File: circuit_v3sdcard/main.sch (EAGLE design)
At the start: 20 parts, among them CN1 SD, CN3 MICROSD, CN4 5035481020, IC1 C8051F381-GM, IC3 N25Q512A, IC4 KC2016K, IC6 MPU-9250

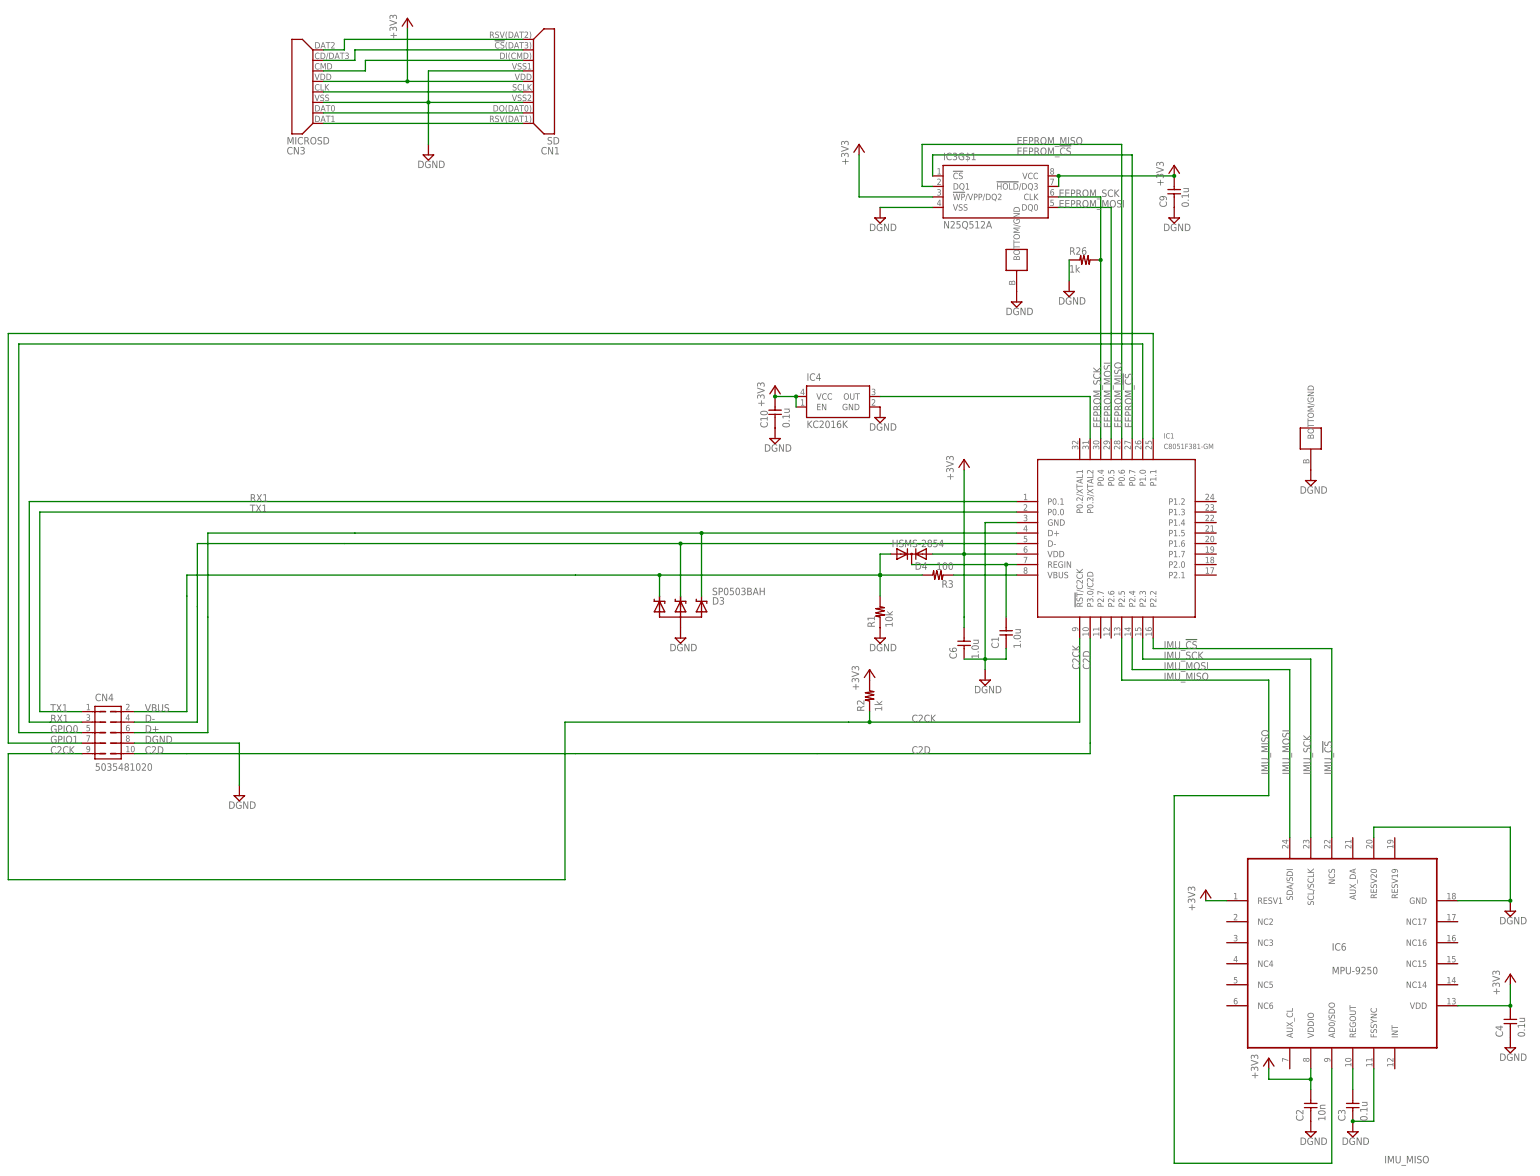
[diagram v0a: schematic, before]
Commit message: Added wiring
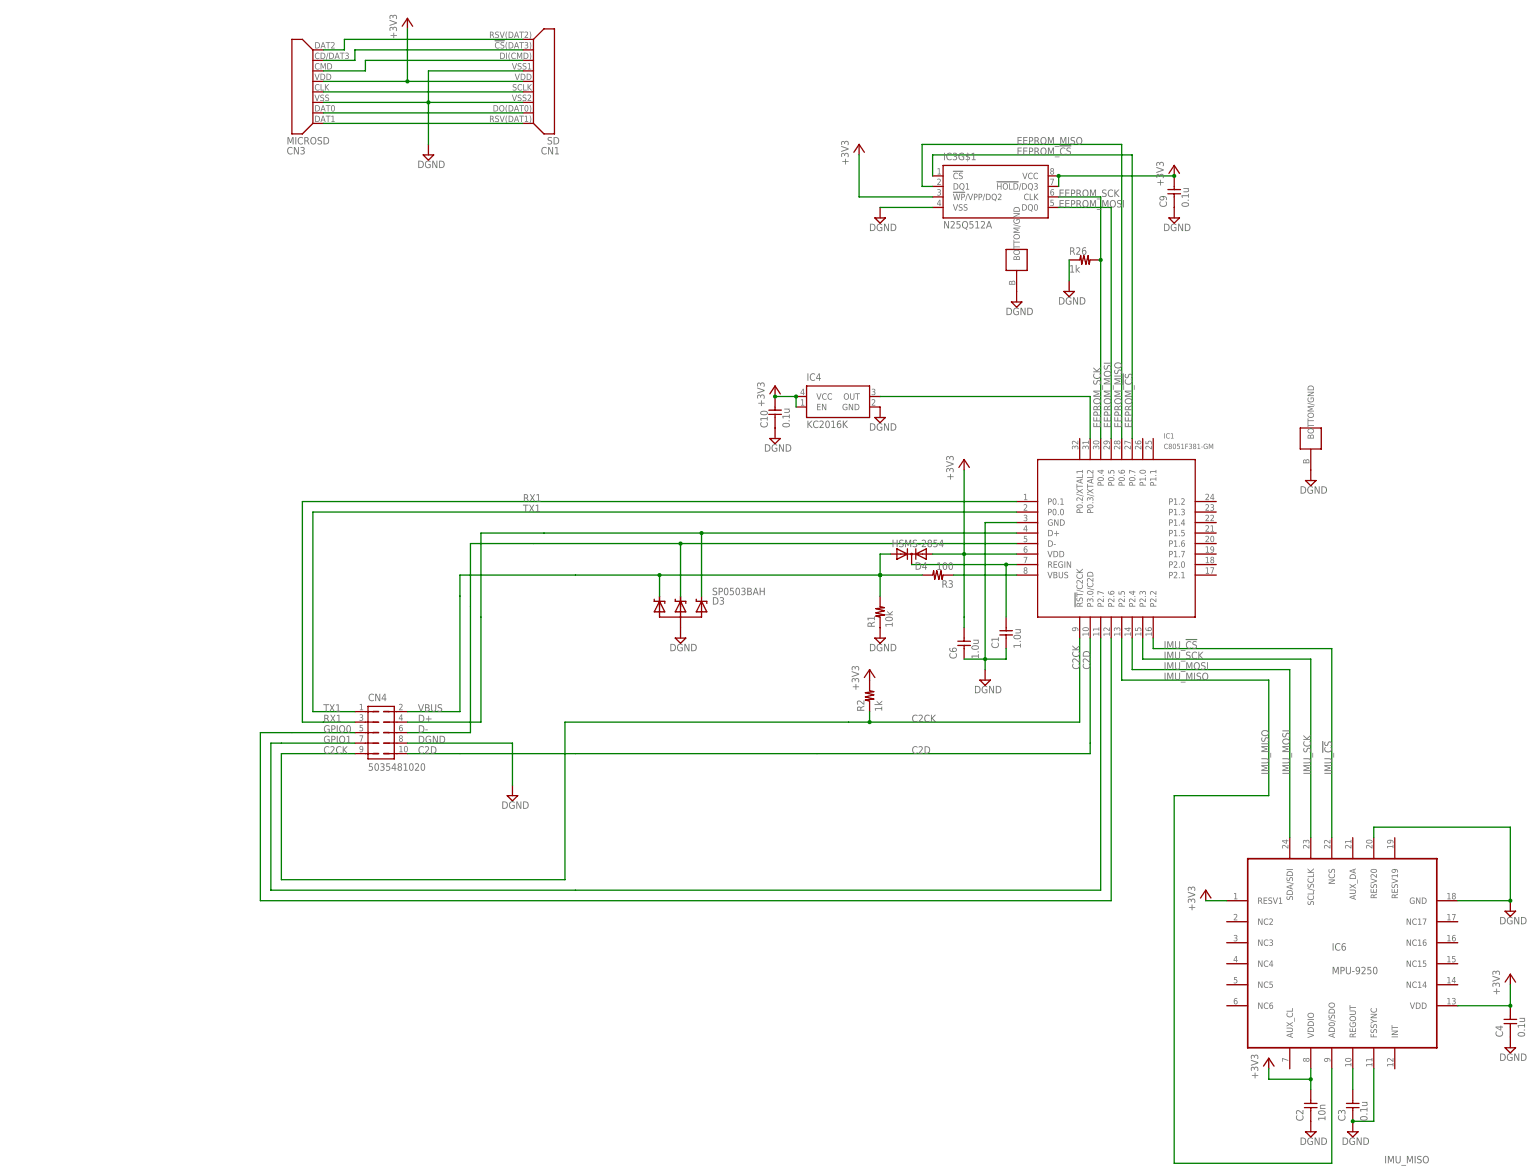
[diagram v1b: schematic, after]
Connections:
- net D+: now also CN4.4; no longer CN4.6
- net D-: now also CN4.6; no longer CN4.4
- net GPIO0: now also IC1G$1.P2.6; no longer IC1G$1.P1.0
- net GPIO1: now also IC1G$1.P2.7; no longer IC1G$1.P1.1
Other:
- moved on the sheet: CN4
